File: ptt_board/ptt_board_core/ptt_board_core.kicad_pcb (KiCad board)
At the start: 2 copper layers, 26.4 x 26.4 mm, 12 parts, among them P019 Conn_01x01_Pin, SW1 RKB2SJG250SMTRLFS, U1 SKB369

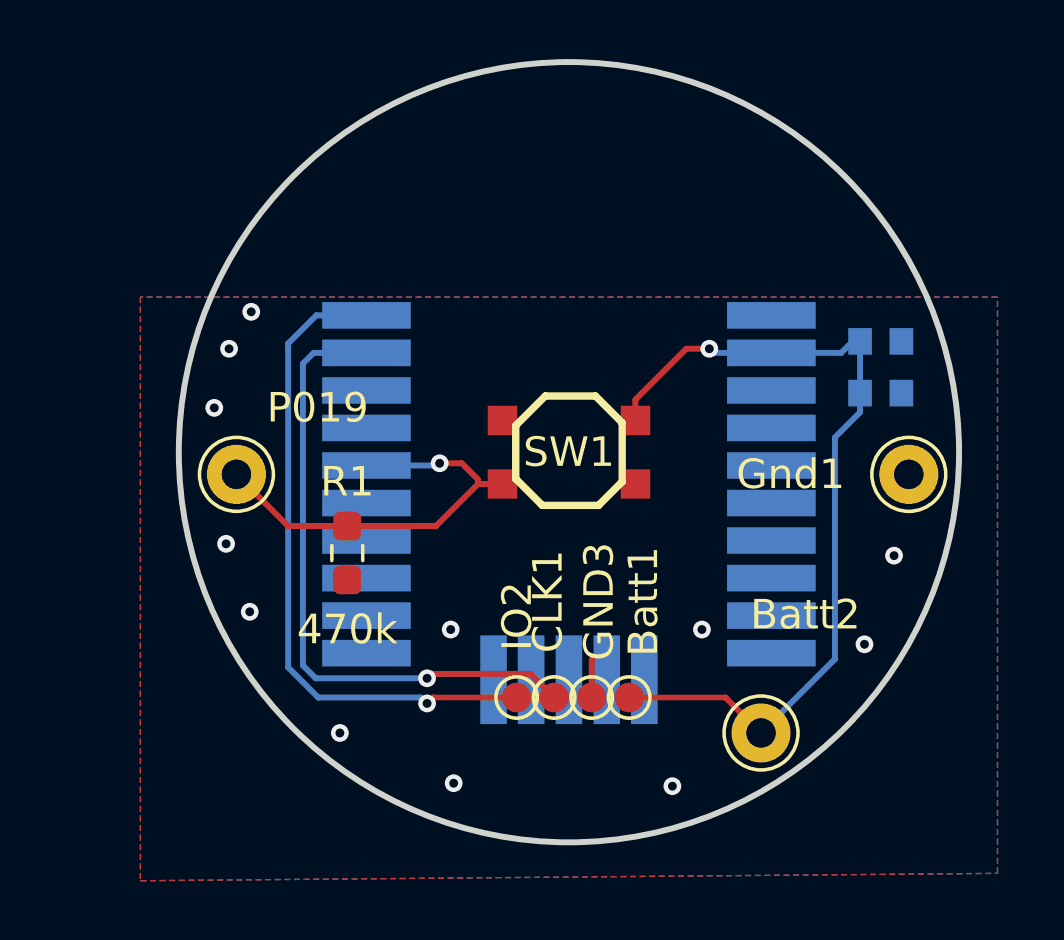
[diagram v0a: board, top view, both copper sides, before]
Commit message: [WIP]
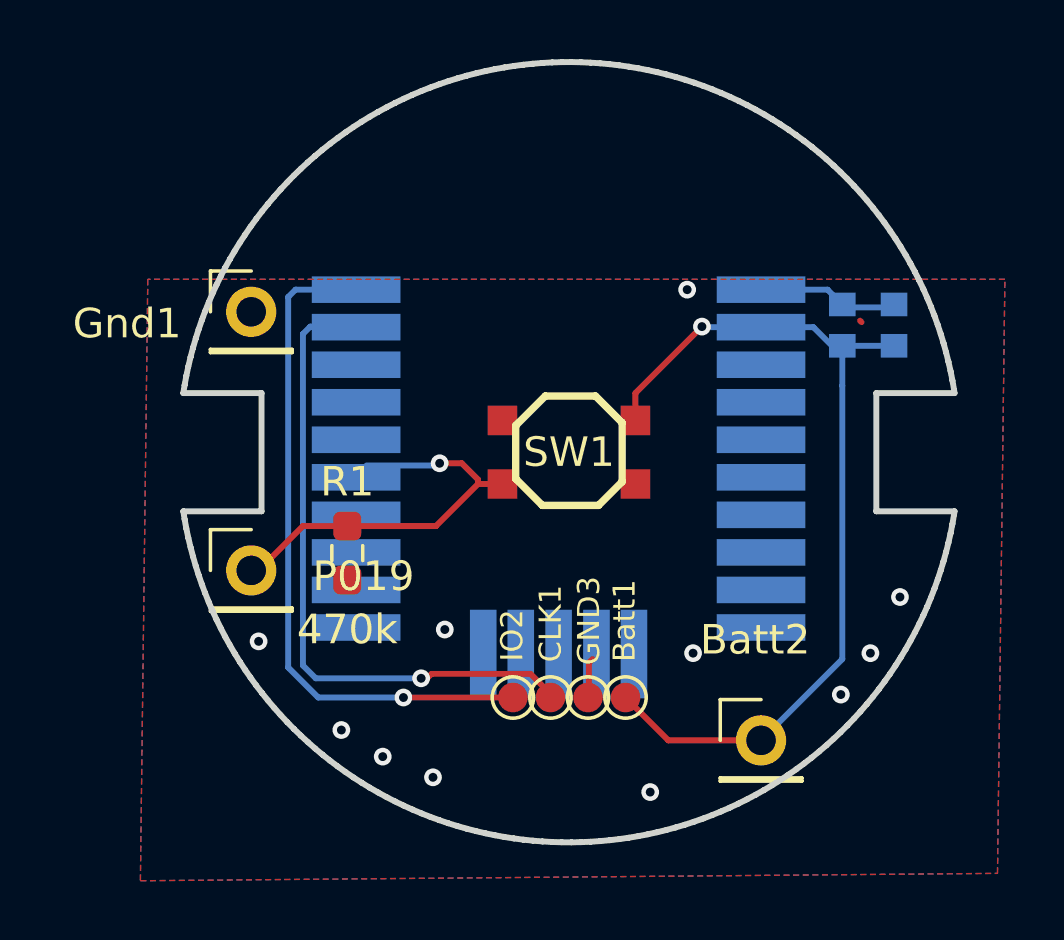
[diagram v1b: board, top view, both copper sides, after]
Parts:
- Batt2, Gnd1, P019: footprint Connector_Pin:Pin_D1.0mm_L10.0mm -> Connector_PinHeader_2.54mm:PinHeader_1x01_P2.54mm_Vertical
- moved Gnd1 22.9 mm to (89.2, 95.2)
- moved P019 3.29 mm to (89.2, 104.0)
- moved C2 2.64 mm to (109.2, 95.7), turned to -90 degrees
- moved U1 0.94 mm to (99.7, 98.1)
- moved C1 0.71 mm to (111.0, 95.7), turned to 90 degrees
- moved Batt2 0.25 mm to (106.5, 109.8)
- moved Batt1 0.12 mm to (101.9, 108.3)
- moved CLK1 0.12 mm to (99.4, 108.3)
- moved GND3 0.12 mm to (100.6, 108.3)
- moved IO2 0.12 mm to (98.1, 108.3)
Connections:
- U1 pad 6: P0.28 -> unconnected-(U1-P0.28-Pad6)
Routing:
- net GND: track 1.31 -> 6.17 mm, vias 12 -> 11
- net P0.19: track 15.0 -> 14.1 mm
- net SWDIO: track 22.3 -> 23.1 mm
- net SWDCLK: track 21.6 -> 22.2 mm
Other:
- board size 26.4 x 26.4 mm -> 26.1 x 26.4 mm
